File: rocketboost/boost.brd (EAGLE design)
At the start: 65 x 30 mm, 18 parts, among them U1 TI61232

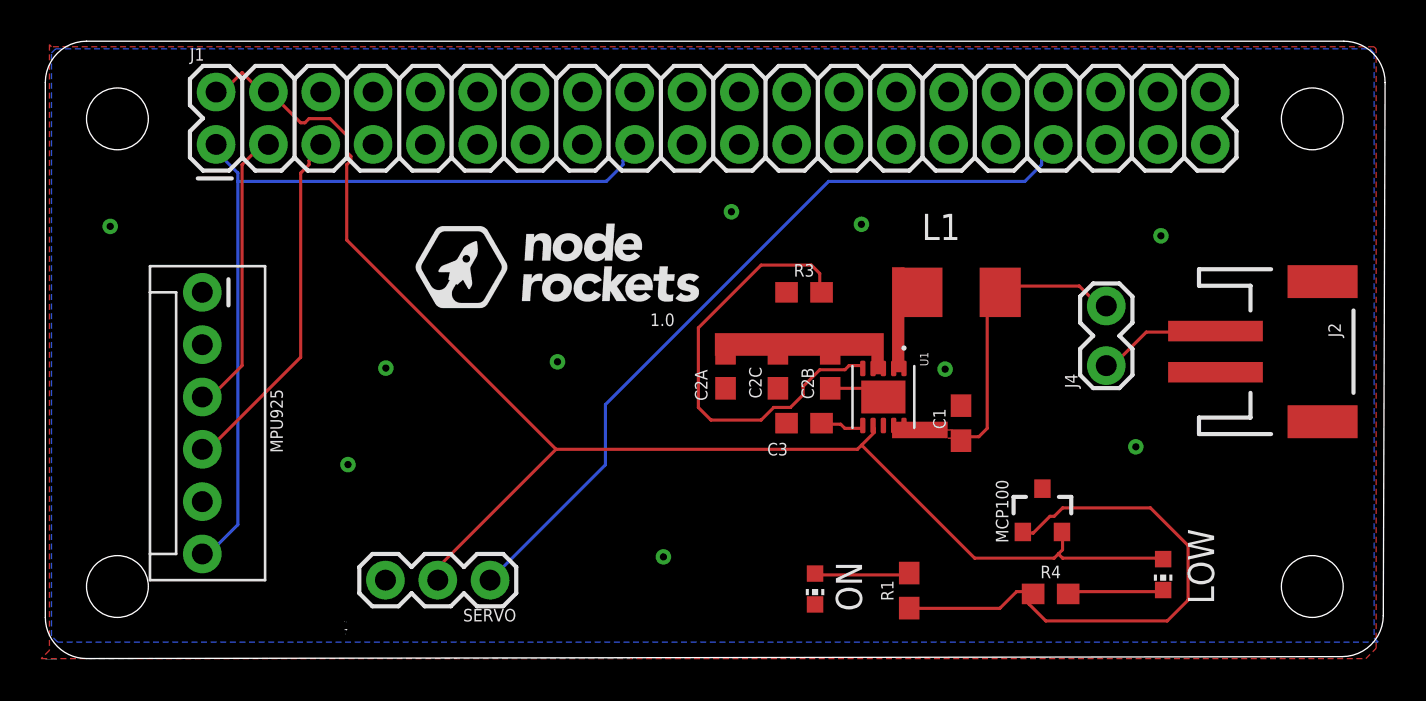
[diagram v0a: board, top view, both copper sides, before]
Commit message: ver 2.0
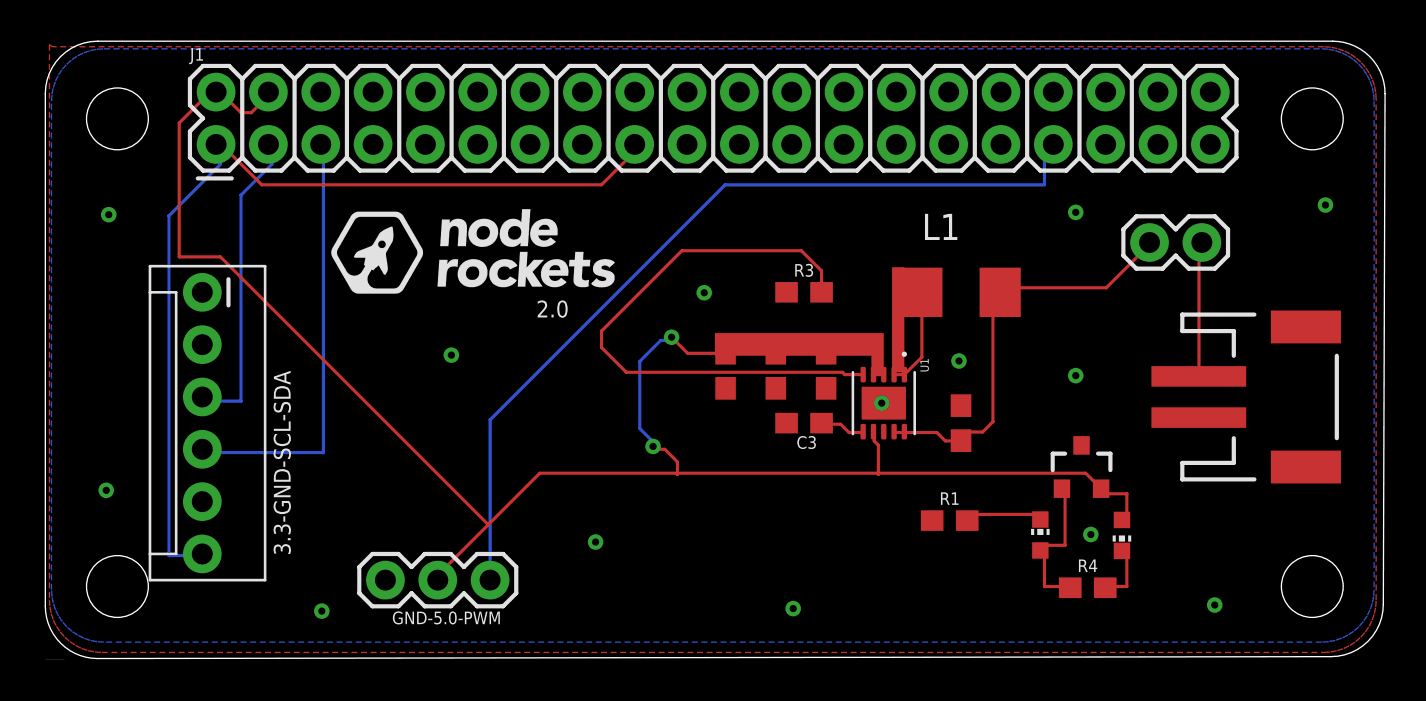
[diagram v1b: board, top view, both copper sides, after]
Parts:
- removed C2B, C2C: 22u, rcl:C0603
- removed J4: (no value), SparkFun-Connectors:1X02_LOCK
- removed LOW, ON: -+, led:CHIP-LED0603
- added C2-B, C2-C: 22uF, rcl:C0603
- added J3: SWITCH, SparkFun-Connectors:1X02
- added LED1: LO, led:CHIP-LED0603
- added LED2: ok, led:CHIP-LED0603
- C2-A: value 22u -> 22uF
- J2: value (none) -> PWR
- U1: value TI61232 -> TPS61232DRCR; device TPS61232DRCR-1:SON50P300X300X100-10N -> steveo:SON50P300X300X100-10N
- moved R1 3.93 mm to (43.9, 6.70), turned to 0 degrees
- moved MCP100 2.83 mm to (50.3, 9.25)
- moved J2 2.34 mm to (59.7, 12.7)
- moved R4 1.82 mm to (50.6, 3.44)
- moved U1 0.30 mm to (40.7, 12.4)
- renumbered C2A to C2-A, MPU925 to 3.3-GND-SCL-SDA, SERVO to GND-5.0-PWM
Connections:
- net PWM renamed N$9
- removed net N$2: ON.A, R1.2
- new net N$22: J2.1, J3.2
- net GND: now also C2-B.2, C2-C.2, R1.1; no longer C2B.2, C2C.2, ON.C
- net N$1: now also LED2.C, R1.2; no longer J2.1, J4.1
- net N$13: now also LED1.C; no longer LOW.C
- net N$4: now also LED2.A; no longer R1.1
- net VIN: now also J3.1; no longer J4.2
- net VOUT: now also C2-B.1, C2-C.1, LED1.A; no longer C2B.1, C2C.1, LOW.A
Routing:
- net VOUT: track 71.0 -> 93.7 mm, vias 0 -> 2
- net N$4: track 27.4 -> 7.19 mm
- net N$22: track 0.00 -> 6.54 mm
- net VIN: track 14.1 -> 20.5 mm
- net PG: track 21.8 -> 27.8 mm
- net SW: track 0.00 -> 4.85 mm
- net N$2: track 4.66 -> 0.00 mm
- net SCL: track 17.4 -> 20.9 mm
- net N$9: track 38.1 -> 41.5 mm
- net V33: track 41.6 -> 44.9 mm
- net N$1: track 5.98 -> 3.78 mm
- net GND: track 1.97 -> 0.00 mm, vias 10 -> 14
- net N$13: track 4.72 -> 2.91 mm
- net SDA: track 14.1 -> 15.0 mm
- removed copper zone on layer 1, net VIN
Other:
- outline, holes or cut-outs redrawn
- board text added: "/Users/olsonsd/Documents/EAGLE/projects/rocketboost/node-rockets.BMP"
- board text added: "2.0"
- board text removed: "/Users/olsonsd/Downloads/node-rockets.BMP"
- board text removed: "1.0"
- board text removed: "BLACK (-)"
- board text removed: "GND 5V PWM"
- board text removed: "RED (+)"
- board text removed: "SDA SCL GND 3.3V"
